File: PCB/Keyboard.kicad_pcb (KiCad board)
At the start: 2 copper layers, 28 x 18 mm, 33 parts, among them J1 RESET, J2 SCK, J3 MISO, J4 MOSI, J5 VBUS, J6 5V, J7 D-, J8 D+, J9 GND, P1 USB_OTG, SW1 RESET, U1 ATMEGA32U4-QFN44, X1 ABM10-16.000MHZ-D30-T3

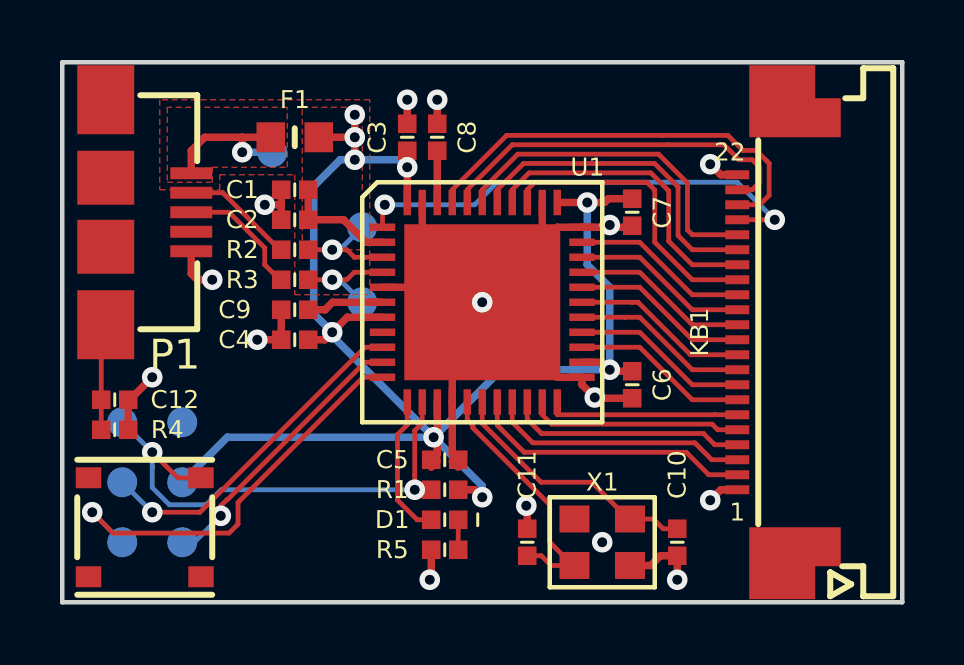
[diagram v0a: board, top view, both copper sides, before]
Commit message: Version 1.3 produced
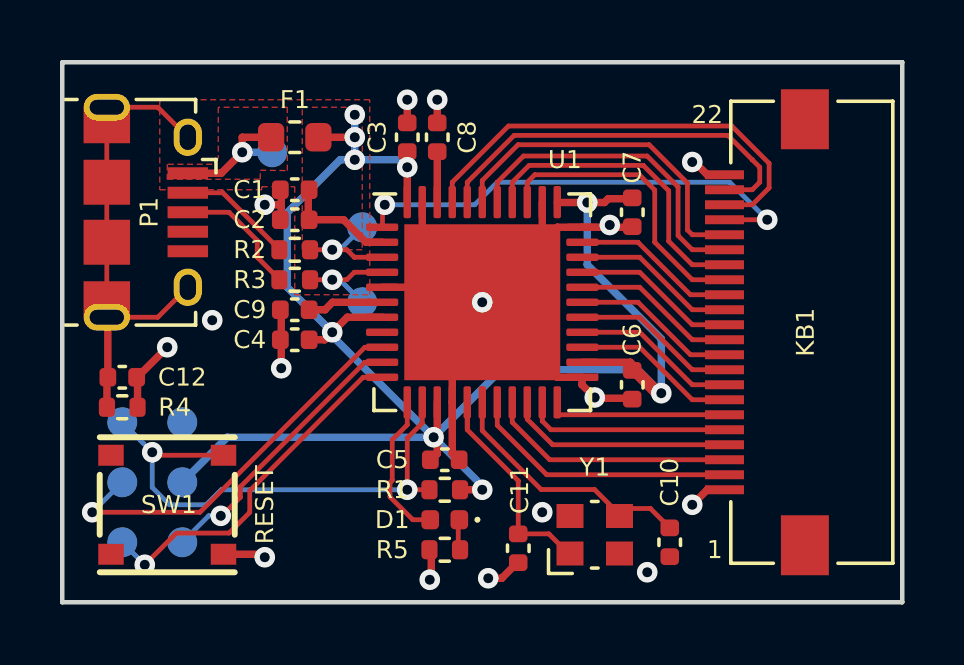
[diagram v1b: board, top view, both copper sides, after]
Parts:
- removed X1: ABM10-16.000MHZ-D30-T3, RB-SMD-XTAL:2.5x2mm
- added Y1: 16MHz, Crystal:Crystal_SMD_Abracon_ABM10-4Pin_2.5x2.0mm, F.Cu at (166.8, 113.8)
- C1, C9: value 1µ -> 1uF; footprint RB-SMD-DiscreteB:C-0402-1005 -> Capacitor_SMD:C_0402_1005Metric
- C10, C11: value 15p -> 6.2pF; footprint RB-SMD-DiscreteB:C-0402-1005 -> Capacitor_SMD:C_0402_1005Metric
- C12: value 4n7 -> 4.7nF; footprint RB-SMD-DiscreteB:C-0402-1005 -> Capacitor_SMD:C_0402_1005Metric
- C2, C3, C4, C5, C6, C7, C8: value 100n -> 100nF; footprint RB-SMD-DiscreteB:C-0402-1005 -> Capacitor_SMD:C_0402_1005Metric
- D1: footprint RB-SMD-DiscreteB:LED-0402-1005 -> LED_SMD:LED_0402_1005Metric
- F1: footprint RB-SMD-DiscreteB:F-0603-1608 -> Fuse:Fuse_0603_1608Metric
- KB1: footprint RB-SMD-Connectors:FPC_0.5mm_22p-MOLEX_52437 -> USB-Keyboard-Adapter-LIBRARY:FPC_22p-JUSHUO_AFC01-S22FCC-00
- P1: footprint RB-SMD-Connectors:USB-MICRO-10104110-0001LF -> Connector_USB:USB_Micro-B_Amphenol_10118194_Horizontal
- R1, R2, R3, R4, R5: footprint RB-SMD-DiscreteB:R-0402-1005 -> Resistor_SMD:R_0402_1005Metric
- U1: footprint RB-SMD-QFN:VQFN-44_ATMEL -> Package_DFN_QFN:QFN-44-1EP_7x7mm_P0.5mm_EP5.2x5.2mm
- moved P1 2.78 mm to (151.8, 103.0)
- moved SW1 1.06 mm to (152.5, 112.8)
- moved C12 0.79 mm to (151.0, 108.5)
- moved R4 0.79 mm to (151.0, 109.5)
- moved KB1 0.43 mm to (171.1, 107.0)
- moved C11 0.36 mm to (164.2, 114.2), turned to -90 degrees
- moved C10 0.25 mm to (169.2, 114.0)
- turned U1 to 0 degrees
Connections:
- P1 pad 4: Net-(P1-Pad4) -> unconnected-(P1-Pad4)
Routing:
- net GNDPWR: track 3.76 -> 16.2 mm
- net GND: track 45.5 -> 36.1 mm, vias 15 -> 16
- net +5V: track 56.7 -> 62.8 mm
- net /SCK: track 11.4 -> 13.4 mm
- net /MISO: track 14.0 -> 12.0 mm
- net /COL_8: track 6.60 -> 5.57 mm
- net /ROW_01: track 12.5 -> 13.3 mm
- net Net-(C11-Pad1): track 8.67 -> 7.98 mm
- net /ROW_08: track 14.4 -> 15.1 mm
- net /RESET: track 17.3 -> 17.9 mm
- net VBUS: track 5.09 -> 4.55 mm
- net /ROW_05: track 10.3 -> 9.81 mm
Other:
- net class Default removed
- net class Power removed
- rule pad_to_mask_clearance: 0.05 -> 0
- board text added: "USB Keyboard v1.3 RasmusB 2022 Psion Series 5/5mx"
- board text removed: "USB Keyboard v1.22 RasmusB 2018 Psion Series 5/5mx"
